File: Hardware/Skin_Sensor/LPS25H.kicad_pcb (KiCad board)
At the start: 2 copper layers, 55 x 55 mm, 49 parts, among them SW1 SW_PUSH, U1 ADP7102, U2 ATSAMD21E18A, U3 AVRISP, U4 LSM9DS1, U5 LP5521YQ, X1 ABS06

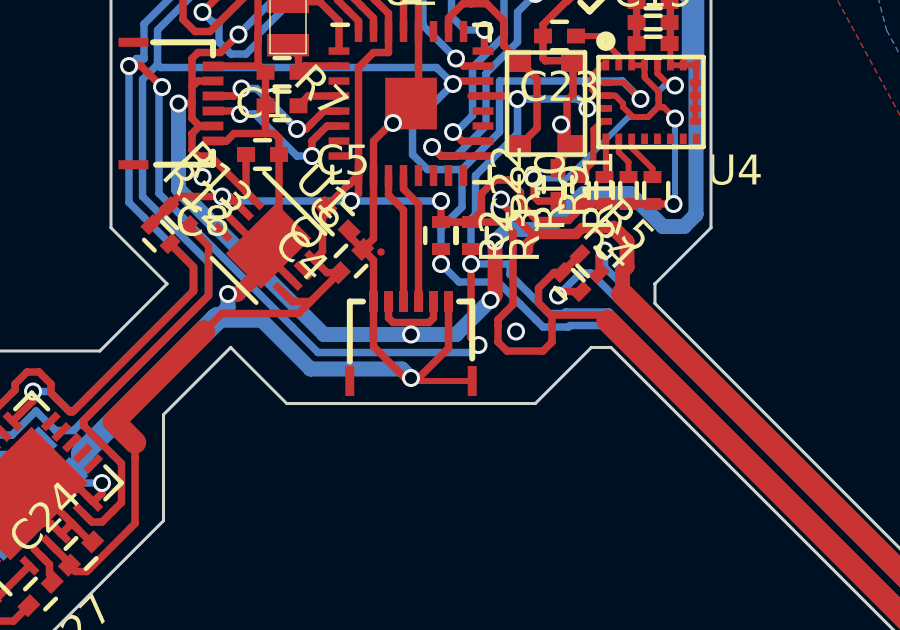
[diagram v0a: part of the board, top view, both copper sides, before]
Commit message: Fixed pour issues
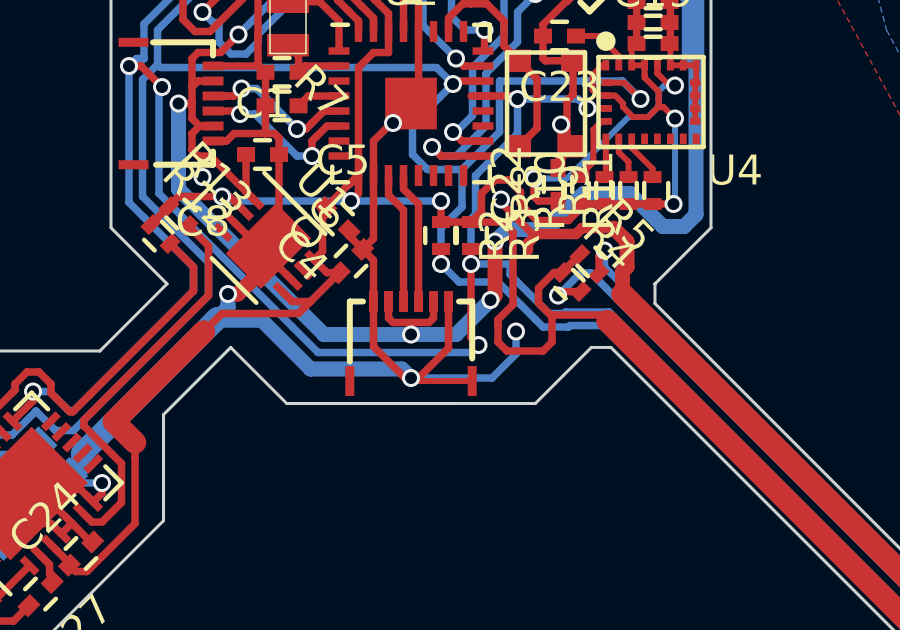
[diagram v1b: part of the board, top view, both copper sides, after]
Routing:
- net GND: track 196.5 -> 200.9 mm, vias 12 -> 11
- net (no net): track 0.32 -> 0.37 mm, vias 0 -> 1
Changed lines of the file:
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@@
     (links 162)
     (no_connects 0)
-    (area 130.545445 70.825409 205.880001 129.245302)
+    (area 123.2 69.2 205.880001 130.350001)
     (thickness 1.6)
     (drawings 91)
@@
   (segment (start 159.172703 87.557501) (end 159.172703 87.840344) (width 0.25) (layer B.Cu) (net 0))
   (segment (start 159.137348 88.47674) (end 159.137348 88.512095) (width 0.25) (layer B.Cu) (net 0))
-  (segment (start 158.9984 104.9484) (end 159 104.95) (width 0.25) (layer F.Cu) (net 0))
+  (segment (start 153.05 102.5) (end 153.05 102.45) (width 0.2) (layer F.Cu) (net 0))
+  (via (at 153.05 102.45) (size 0.6) (drill 0.4) (layers F.Cu B.Cu) (net 0))
   (segment (start 165.75 103) (end 164.55 104.2) (width 0.5) (layer B.Cu) (net 1))
   (via (at 165.3 94.65) (size 0.6) (drill 0.4) (layers F.Cu B.Cu) (net 1))
@@
   (segment (start 158.394885 81.053514) (end 158.394885 85.05) (width 0.25) (layer F.Cu) (net 1))
   (segment (start 158.394885 85.05) (end 158.394885 85.082627) (width 0.25) (layer F.Cu) (net 1))
-  (segment (start 163.6 107.55) (end 163.55 107.6) (width 0.25) (layer B.Cu) (net 2))
+  (segment (start 160 109.15) (end 162.7 109.15) (width 0.25) (layer B.Cu) (net 2))
   (via (at 163.5 107.6) (size 0.6) (drill 0.4) (layers F.Cu B.Cu) (net 2))
-  (segment (start 163.55 107.6) (end 163.5 107.6) (width 0.25) (layer B.Cu) (net 2))
-  (segment (start 164.9 102.15) (end 165 102.05) (width 0.25) (layer F.Cu) (net 2) (status C00000))
-  (segment (start 165 102.05) (end 165 100.7) (width 0.25) (layer F.Cu) (net 2) (status 400000))
+  (segment (start 163.5 108.35) (end 163.5 107.6) (width 0.25) (layer B.Cu) (net 2))
+  (segment (start 162.7 109.15) (end 163.5 108.35) (width 0.25) (layer B.Cu) (net 2))
+  (segment (start 164.9 102.15) (end 165 102.05) (width 0.25) (layer F.Cu) (net 2))
+  (segment (start 165 102.05) (end 165 100.7) (width 0.25) (layer F.Cu) (net 2))
   (via (at 165 100.7) (size 0.6) (drill 0.4) (layers F.Cu B.Cu) (net 2))
-  (segment (start 165.4 101.425) (end 164.9 101.925) (width 0.25) (layer F.Cu) (net 2) (status C00000))
-  (segment (start 164.9 101.925) (end 164.9 102.15) (width 0.25) (layer F.Cu) (net 2) (status C00000))
+  (segment (start 165.4 101.425) (end 164.9 101.925) (width 0.25) (layer F.Cu) (net 2))
+  (segment (start 164.9 101.925) (end 164.9 102.15) (width 0.25) (layer F.Cu) (net 2))
   (segment (start 164.175 104.375) (end 164.075 104.375) (width 0.25) (layer F.Cu) (net 2))
   (via (at 163 103.2) (size 0.6) (drill 0.4) (layers F.Cu B.Cu) (net 2))
   (segment (start 163 103.3) (end 163 103.2) (width 0.25) (layer F.Cu) (net 2))
   (segment (start 164.075 104.375) (end 163 103.3) (width 0.25) (layer F.Cu) (net 2))
-  (via (at 159.4 100.65) (size 0.6) (drill 0.4) (layers F.Cu B.Cu) (net 2) (status 800000))
-  (segment (start 159.4 100.65) (end 160 100.05) (width 0.2) (layer F.Cu) (net 2) (status C00000))
-  (segment (start 160 100.05) (end 160 100) (width 0.2) (layer F.Cu) (net 2) (status C00000))
-  (segment (start 153.05 102.5) (end 153.05 102.45) (width 0.2) (layer F.Cu) (net 2))
-  (via (at 153.05 102.45) (size 0.6) (drill 0.4) (layers F.Cu B.Cu) (net 2))
+  (via (at 159.4 100.65) (size 0.6) (drill 0.4) (layers F.Cu B.Cu) (net 2))
+  (segment (start 159.4 100.65) (end 160 100.05) (width 0.2) (layer F.Cu) (net 2))
+  (segment (start 160 100.05) (end 160 100) (width 0.2) (layer F.Cu) (net 2))
   (segment (start 162.04 109.25) (end 160.1 109.25) (width 0.2) (layer F.Cu) (net 2))
   (via (at 160 109.15) (size 0.6) (drill 0.4) (layers F.Cu B.Cu) (net 2))
@@
   (segment (start 162.8 102.55) (end 163.25 102.55) (width 0.25) (layer F.Cu) (net 3))
   (segment (start 163.25 102.55) (end 163.65 102.95) (width 0.25) (layer F.Cu) (net 3))
-  (segment (start 162.35 103.6) (end 162 103.95) (width 0.25) (layer F.Cu) (net 3) (status 800000))
+  (segment (start 162.35 103.6) (end 162 103.95) (width 0.25) (layer F.Cu) (net 3))
   (segment (start 163.65 103.35) (end 163.65 102.95) (width 0.25) (layer F.Cu) (net 3))
   (segment (start 164.2 103.9) (end 163.65 103.35) (width 0.25) (layer F.Cu) (net 3))
   (segment (start 163.4 106.7) (end 163.4 104.3) (width 0.25) (layer F.Cu) (net 3))
   (segment (start 163.4 104.3) (end 163.05 103.95) (width 0.25) (layer F.Cu) (net 3))
-  (segment (start 163.05 103.95) (end 162 103.95) (width 0.25) (layer F.Cu) (net 3) (status 800000))
+  (segment (start 163.05 103.95) (end 162 103.95) (width 0.25) (layer F.Cu) (net 3))
   (segment (start 162.9 107.4) (end 162.9 107.95) (width 0.25) (layer F.Cu) (net 3))
   (segment (start 163.4 106.7) (end 162.9 107.2) (width 0.25) (layer F.Cu) (net 3))
@@
   (via (at 164.1 102.5) (size 0.6) (drill 0.4) (layers F.Cu B.Cu) (net 41))
   (segment (start 166 101.7) (end 165.2 102.5) (width 0.2) (layer B.Cu) (net 41))
-  (segment (start 164.25 103.25) (end 164.9 103.25) (width 0.25) (layer F.Cu) (net 41) (status 800000))
+  (segment (start 164.25 103.25) (end 164.9 103.25) (width 0.25) (layer F.Cu) (net 41))
   (segment (start 164.1 103.1) (end 164.25 103.25) (width 0.25) (layer F.Cu) (net 41))
   (segment (start 168.215 98.725) (end 168.215 99) (width 0.2) (layer F.Cu) (net 41))
